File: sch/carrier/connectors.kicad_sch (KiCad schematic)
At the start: 2 parts, among them J2 1054500101

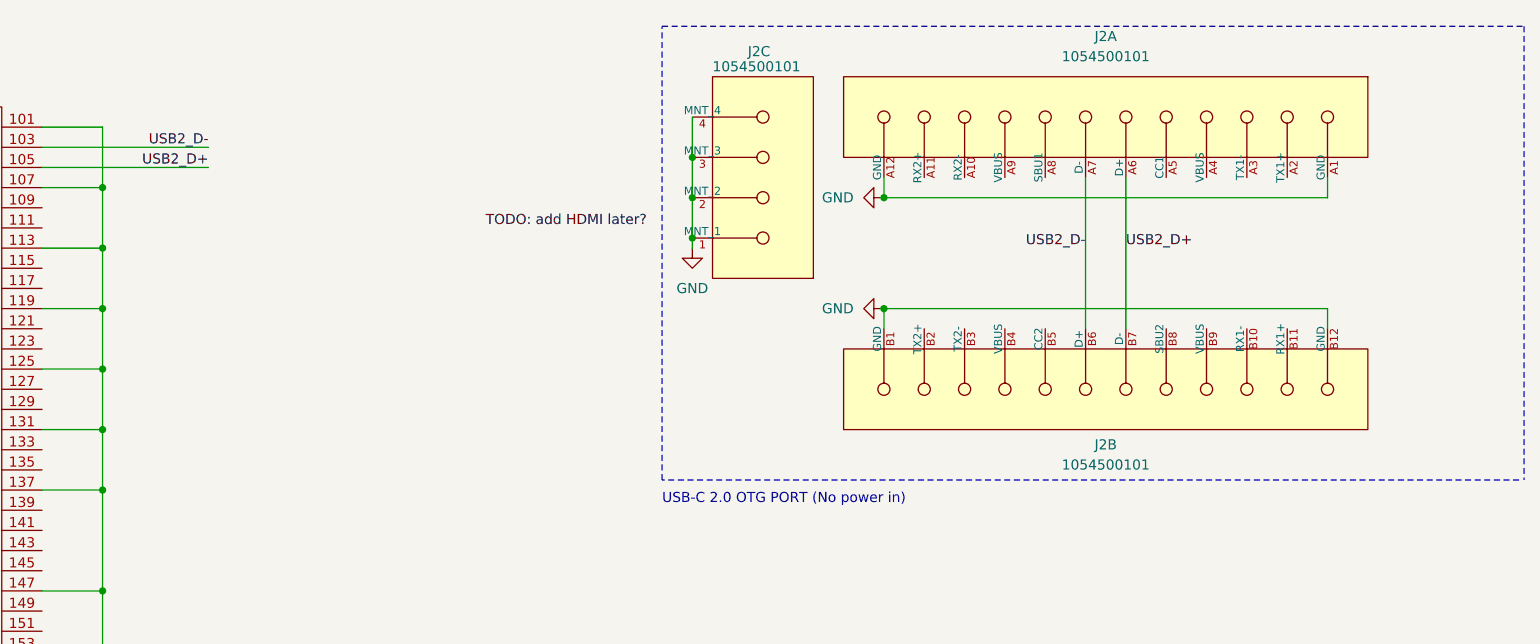
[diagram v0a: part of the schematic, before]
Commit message: a
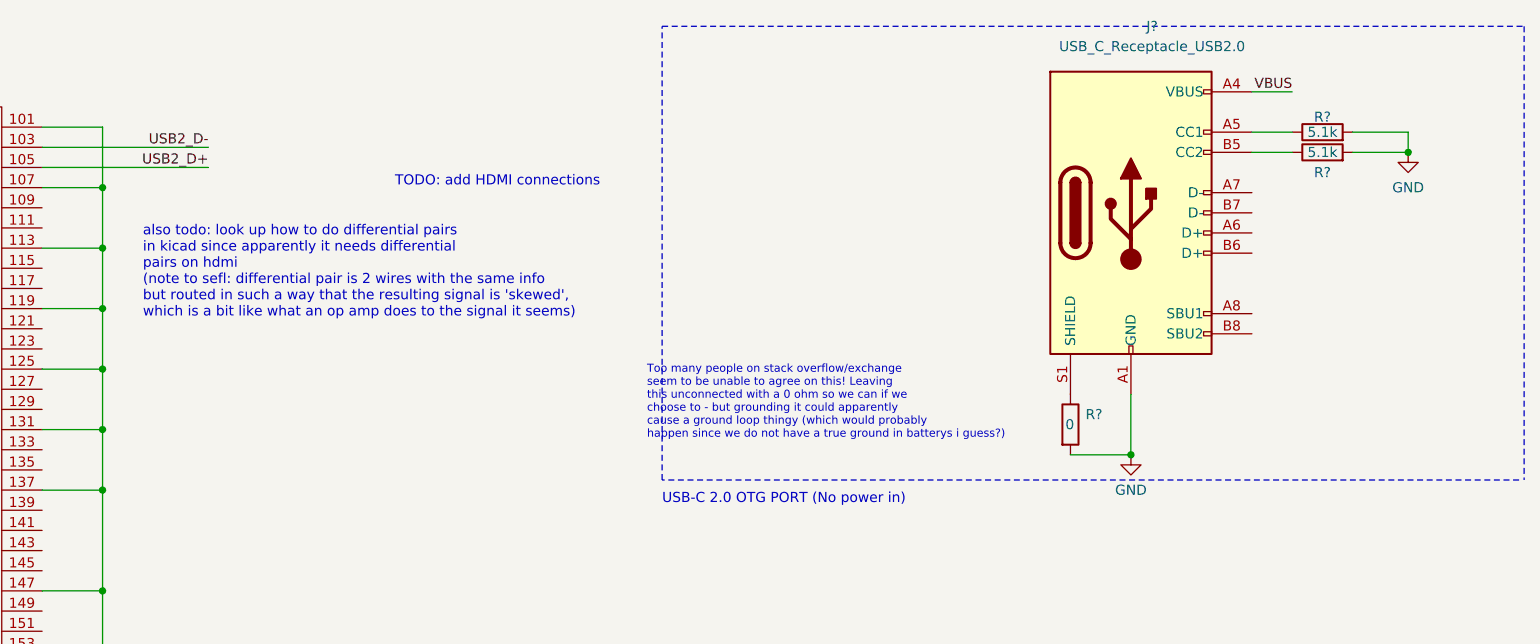
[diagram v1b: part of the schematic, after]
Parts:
- removed J2: 1054500101, MOLEXC:Molex-1054500101-MFG, symbol MOLEXC:1054500101
- added J?: USB_C_Receptacle_USB2.0, Connector_USB:USB_C_Receptacle_JAE_DX07S016JA1R1500, symbol Connector:USB_C_Receptacle_USB2.0
- added R? (x2): 5.1k, Resistor_SMD:R_0805_2012Metric_Pad1.20x1.40mm_HandSolder, symbol Device:R
- added R?: 0, symbol Device:R
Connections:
- net GND: now also J?.A1 (GND), J?.A12 (GND), J?.B1 (GND), J?.B12 (GND), R?.2, R?.2, R?.2
- new net: J?.A5 (CC1), R?.1
- new net: J?.S1 (SHIELD), R?.1
- new net: J?.B5 (CC2), R?.1
- new net VBUS: J?.A4 (VBUS), J?.A9 (VBUS), J?.B4 (VBUS), J?.B9 (VBUS)
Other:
- note added: "TODO: add HDMI connections"
- note added: "Too many people on stack overflow/exchange seem to be unable to agree on this! Leaving this unconnected with a 0 ohm so we can if we choose to - but grounding it could apparently cause a ground loop thingy (which would probably happen since we do not have a true ground in batterys i guess?)"
- note added: "also todo: look up how to do differential pairs in kicad since apparently it needs differential pairs on hdmi (note to sefl: differential pair is 2 wires with the same info but routed in such a way that the resulting signal is 'skewed', which is a bit like what an op amp does to the signal it seems)"
